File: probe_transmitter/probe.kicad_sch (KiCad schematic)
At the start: 20 parts, among them Q1 PMST2222, U1 ATtiny85-20M

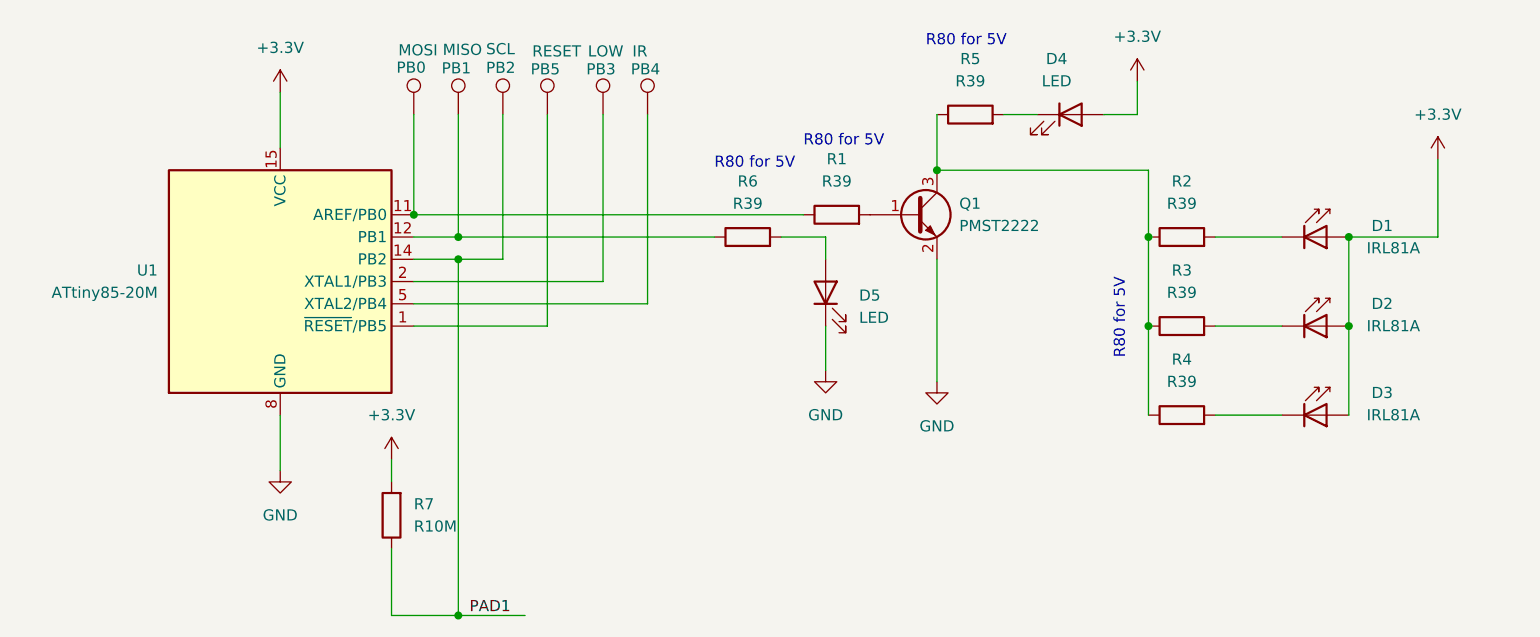
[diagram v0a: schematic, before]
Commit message: - add new power version
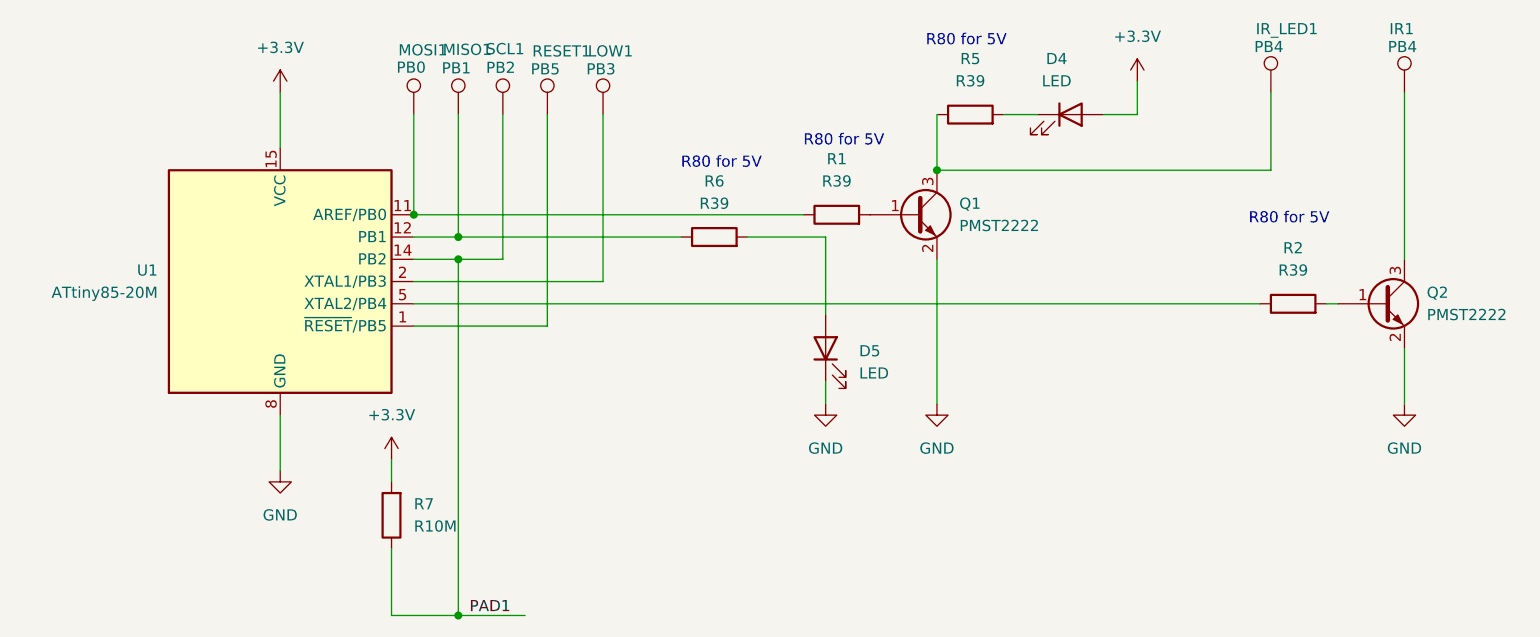
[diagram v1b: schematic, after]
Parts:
- removed D1, D2, D3: IRL81A, LED_THT:LED_SideEmitter_Rectangular_W4.5mm_H1.6mm, symbol LED:IRL81A
- removed R3, R4: R39, Resistor_SMD:R_0603_1608Metric, symbol Device:R
- added IR_LED1: PB4, TestPoint:TestPoint_Pad_D1.0mm, symbol Connector:TestPoint
- added Q2: PMST2222, Package_TO_SOT_SMD:SOT-23, symbol Transistor_BJT:BC817
- renumbered IR to IR1, LOW to LOW1, MISO to MISO1, MOSI to MOSI1, RESET to RESET1, SCL to SCL1
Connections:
- net GND: now also Q2.2 (E)
- net at Q1.3 (C), R5.1: now also IR_LED1.1; no longer R2.1
- net at U1.5 (XTAL2/PB4): now also R2.1; no longer IR1.1
- net at R2.2: now also Q2.1 (B)
- new net: IR1.1, Q2.3 (C)
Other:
- moved on the sheet: D5, IR1, R6
